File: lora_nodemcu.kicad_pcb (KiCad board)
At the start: 4 copper layers, 26 x 43.5 mm, 10 parts, among them U1 RFM95, U2 LM1117-3.3, U3 WeMos_mini

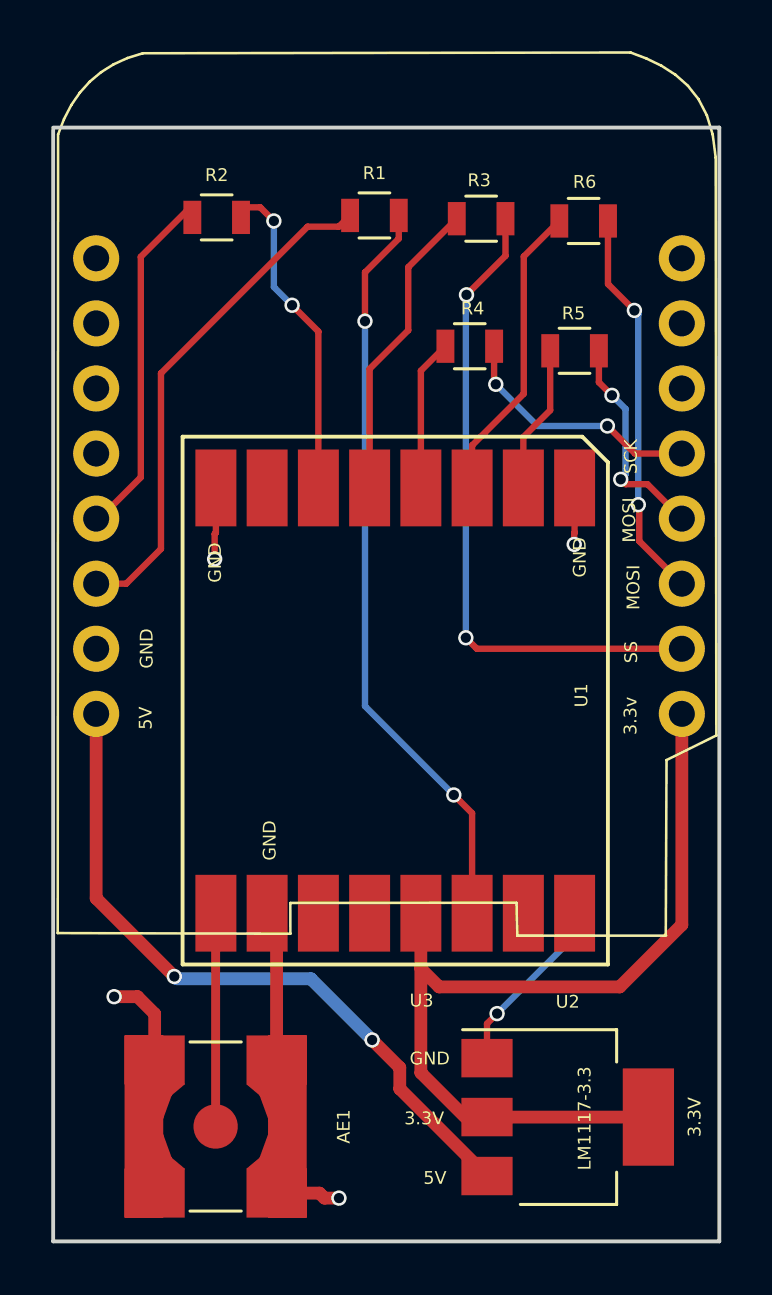
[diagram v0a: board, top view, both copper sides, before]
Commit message: backup save for prosperity
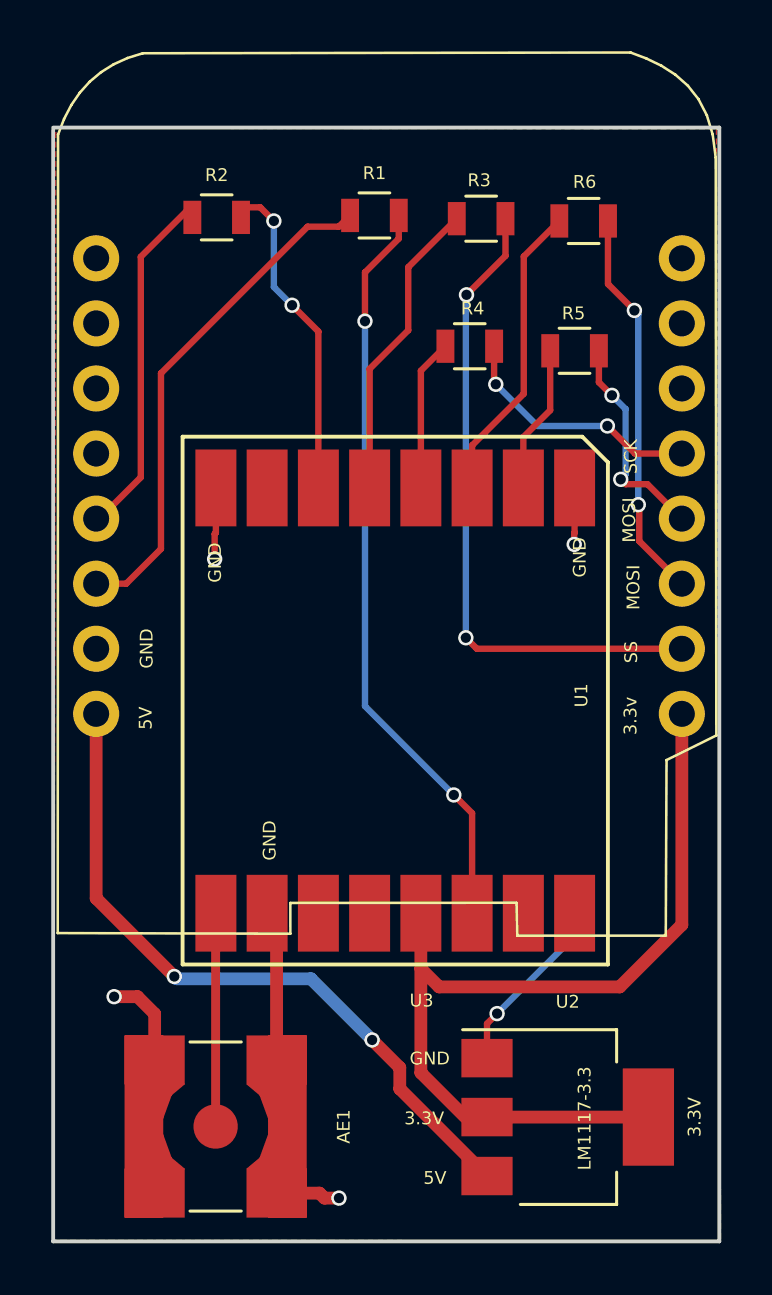
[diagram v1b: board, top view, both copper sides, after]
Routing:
- added copper zone on B.Cu, net GND
- added copper zone on F.Cu, net GND
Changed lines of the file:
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@@
     (links 35)
     (no_connects 0)
-    (area 150.174999 111.049999 176.325001 154.672101)
+    (area 150.174999 107.945765 176.383721 154.872)
     (thickness 1.2)
     (drawings 19)
@@
   (layers
     (0 F.Cu signal)
-    (1 In1.Cu power)
-    (2 In2.Cu power)
-    (31 B.Cu signal)
+    (1 In1.Cu power hide)
+    (2 In2.Cu power hide)
+    (31 B.Cu signal hide)
     (33 F.Adhes user)
     (35 F.Paste user)
@@
   )
   (setup
-    (last_trace_width 0.5)
+    (last_trace_width 0.25)
     (user_trace_width 0.5)
     (trace_clearance 0.2)
@@
     (effects (font (size 0.5 0.5) (thickness 0.1)))
   )
-  (gr_text GND (at 164.9476 147.4597 360) (layer F.SilkS)
+  (gr_text GND (at 164.9476 147.4597) (layer F.SilkS)
     (effects (font (size 0.5 0.5) (thickness 0.1)))
   )
@@
       )
     )
+  )
+  (zone (net 15) (net_name GND) (layer F.Cu) (hatch edge 0.508)
+    (connect_pads (clearance 0.1524))
+    (min_thickness 0.254)
+    (fill yes (arc_segments 16) (thermal_gap 0.508) (thermal_bridge_width 0.508))
+    (polygon
+      (pts
+        (xy 150.3553 111.1504) (xy 176.1363 111.1758) (xy 176.3014 154.6225) (xy 150.2664 154.6225)
+      )
+    )
+  )
+  (zone (net 15) (net_name GND) (layer B.Cu) (hatch edge 0.508)
+    (connect_pads (clearance 0.1524))
+    (min_thickness 0.254)
+    (fill yes (arc_segments 16) (thermal_gap 0.508) (thermal_bridge_width 0.508))
+    (polygon
+      (pts
+        (xy 150.241 111.125) (xy 176.2252 111.1504) (xy 176.2506 154.5717) (xy 150.2537 154.559)
+      )
+    )
+  )
+  (zone (net 0) (net_name "") (layer F.Cu) (hatch edge 0.508)
+    (connect_pads (clearance 0.1524))
+    (min_thickness 0.254)
+    (keepout (tracks allowed) (vias allowed) (copperpour not_allowed))
+    (fill yes (arc_segments 16) (thermal_gap 0.508) (thermal_bridge_width 0.508))
+    (polygon
+      (pts
+        (xy 154.9527 143.5862) (xy 158.5849 143.6243) (xy 159.0167 154.4701) (xy 154.8511 154.4955) (xy 154.9527 143.6116)
+      )
+    )
